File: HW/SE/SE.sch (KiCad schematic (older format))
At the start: 17 parts, among them J1 Conn_01x03_Female, SW1 SW_Push, SW2 Reset, U1 ESP32-WROOM-32, U2 NHD-0420H1Z, U3 NHD-0420H1Z, U4 PCF8574

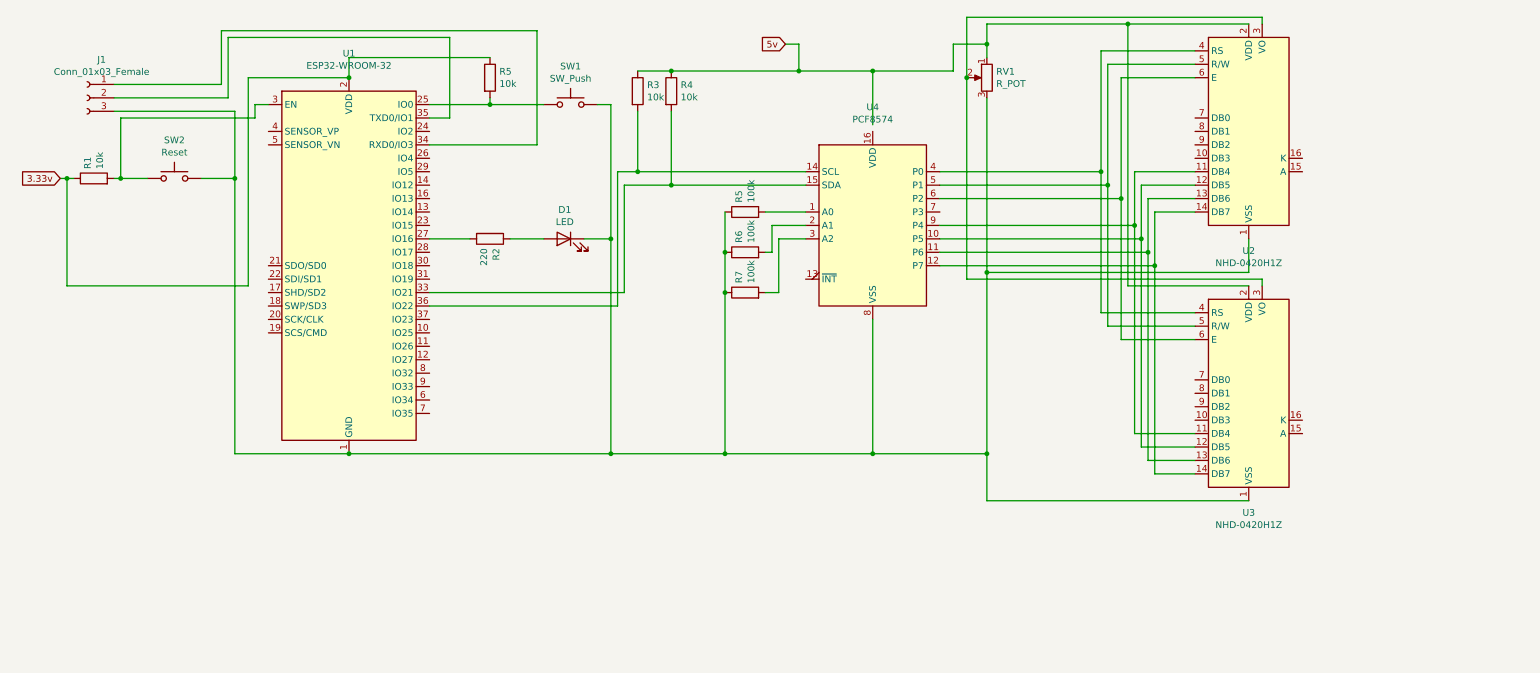
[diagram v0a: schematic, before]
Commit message: AJustes Dsiplay
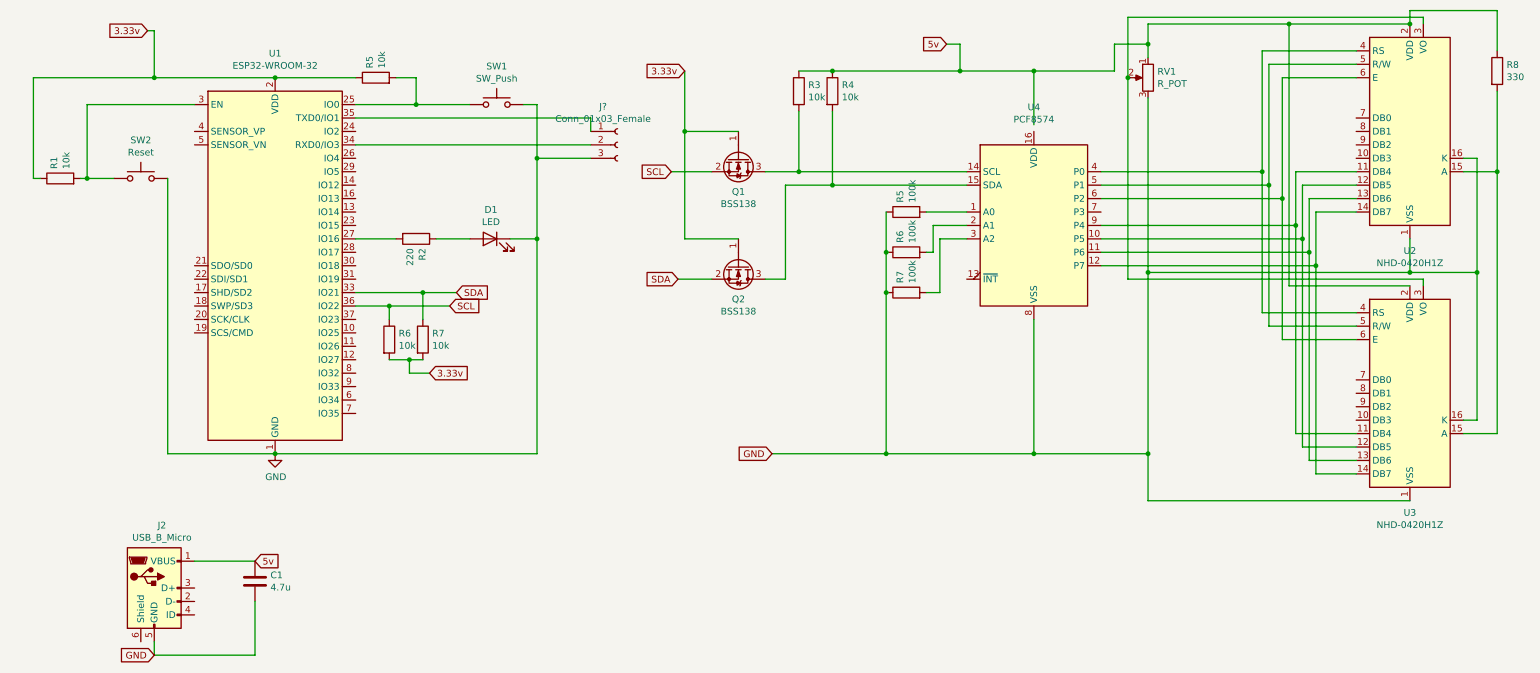
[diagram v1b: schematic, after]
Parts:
- removed J1: Conn_01x03_Female, symbol Connector:Conn_01x03_Female
- added C1: 4.7u, symbol Device:C
- added J2: USB_B_Micro, symbol Connector:USB_B_Micro
- added J?: Conn_01x03_Female, symbol Connector:Conn_01x03_Female
- added Q1, Q2: BSS138, Package_TO_SOT_SMD:SOT-23, symbol Transistor_FET:BSS138
- added R6, R7: 10k, symbol Device:R
- added R8: 330, symbol Device:R
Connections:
- net 3.33v: now also Q1.1 (G), Q2.1 (G), R6.2, R7.2
- net 5v: now also C1.1, J2.1 (VBUS), R8.1
- net GND: now reaches D1.1 (K), R5.1, R6.1, R7.1, RV1.3, SW1.2, SW2.2, U1.1 (GND), U1.15 (GND), U1.38 (GND), U1.39 (GND), U2.1 (VSS), U3.1 (VSS), U4.8 (VSS)
- net GND: now also U2.16 (K), U3.16 (K), C1.2, J2.5 (GND), J?.3 (Pin_3)
- net at R4.2, U4.15 (SDA): now also Q2.3 (D); no longer U1.33 (IO21)
- net at U1.34 (RXD0/IO3): now also J?.2 (Pin_2)
- net at U1.35 (TXD0/IO1): now also J?.1 (Pin_1)
- net at R3.2, U4.14 (SCL): now also Q1.3 (D); no longer U1.36 (IO22)
- net at U2.15 (A): now also U3.15 (A), R8.2
- new net SCL: Q1.2 (S), R6.1, U1.36 (IO22)
- new net SDA: Q2.2 (S), R7.1, U1.33 (IO21)
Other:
- moved on the sheet: D1, R1, R2, R3, R4, R5, R6, R7, RV1, SW1, SW2, U1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
